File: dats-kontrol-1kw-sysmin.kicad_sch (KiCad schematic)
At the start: 26 parts, among them J1 SWD, J3 USB_B, J7 Conn_01x12, SW1 SW?, U1 AMS1117CD-3.3, U2 STM32F4X1CXU6, Y1 25MHZ 9PF, Y2 32.768KHz

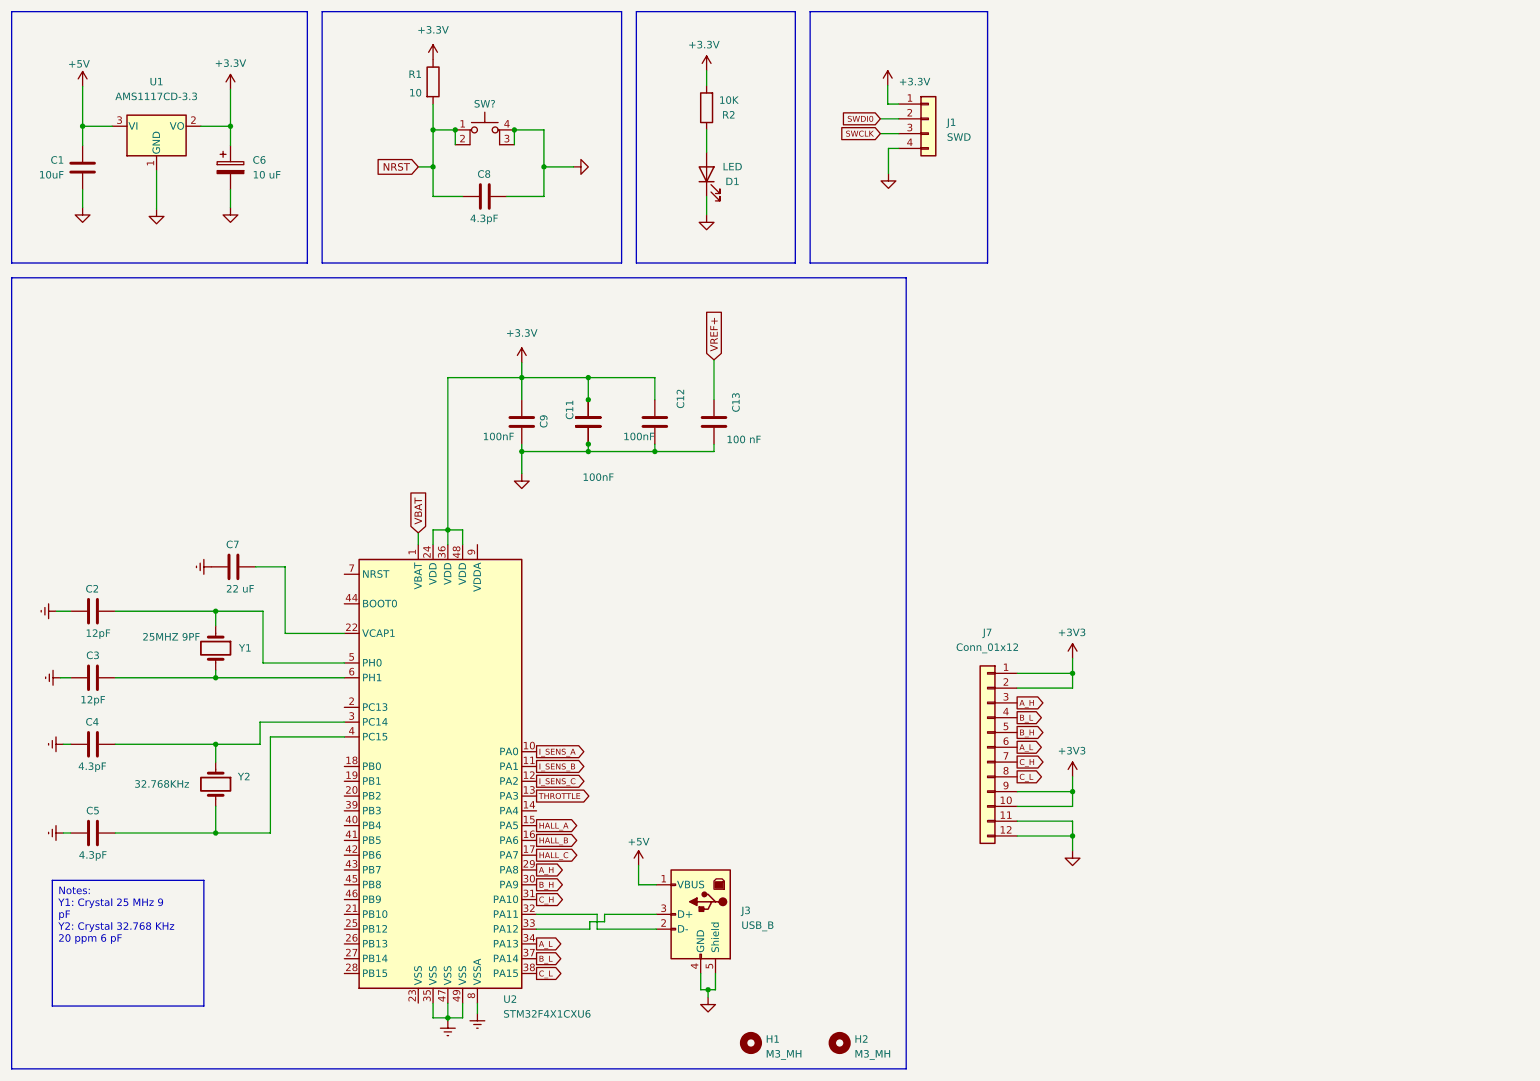
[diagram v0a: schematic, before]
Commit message: new layout
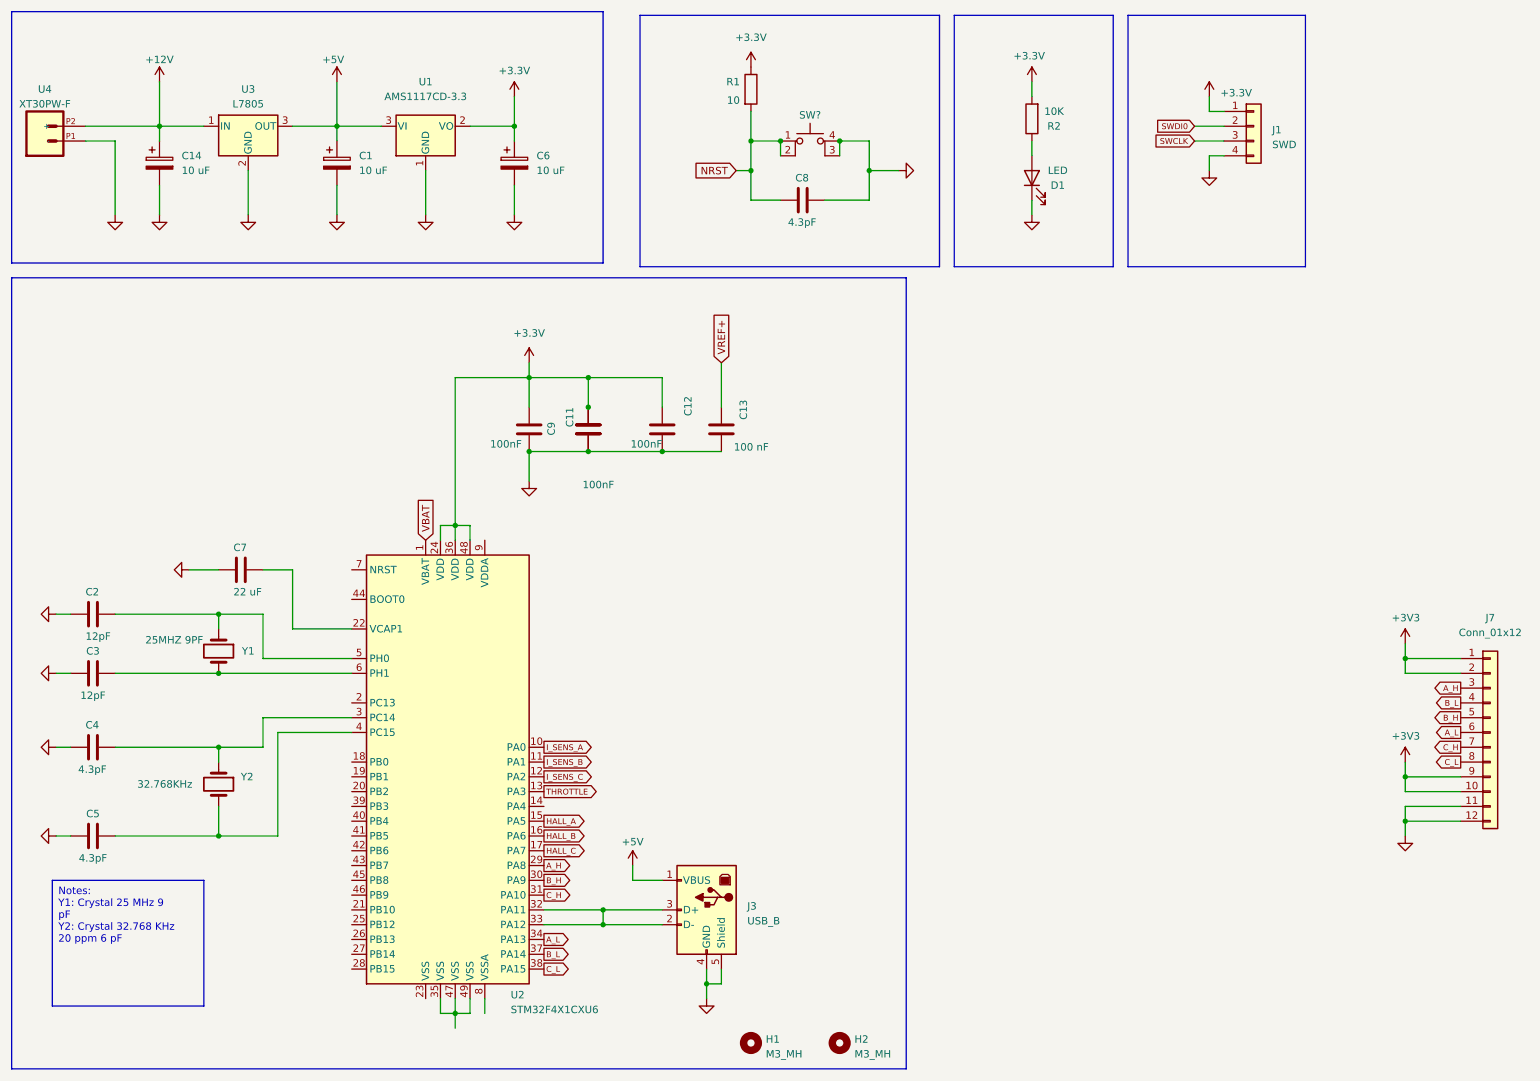
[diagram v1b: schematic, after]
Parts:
- removed C1: 10uF, Capacitor_SMD:C_0805_2012Metric, symbol Device:C
- added C1, C14: 10 uF, Capacitor_SMD:CP_Elec_5x5.3, symbol Device:C_Polarized
- added U3: L7805, Package_TO_SOT_SMD:TO-252-2, symbol Regulator_Linear:L7805
- added U4: XT30PW-F, XT30:XT30PW-F, symbol XT30PW-F:XT30PW-F
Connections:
- net +5V: now also C1.1, U3.3 (OUT)
- net GND: now also C2.2, C3.2, C4.2, C5.2, C7.2, C1.2, C14.2, U3.2 (GND), U4.P1 (-)
- net at J3.2 (D-), U2.32 (PA11): now also J3.3 (D+), U2.33 (PA12)
- removed net Earth: C2.2, C3.2, C4.2, C5.2, C7.2, U2.35 (VSS), U2.47 (VSS), U2.49 (VSS), U2.8 (VSSA)
- new net: U2.35 (VSS), U2.47 (VSS), U2.49 (VSS)
- new net +12V: C14.1, U3.1 (IN), U4.P2 (+)
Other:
- moved on the sheet: C11, C12, C13, C2, C3, C4, C5, C6, C7, C8, C9, D1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
